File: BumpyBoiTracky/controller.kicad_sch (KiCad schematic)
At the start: 9 parts

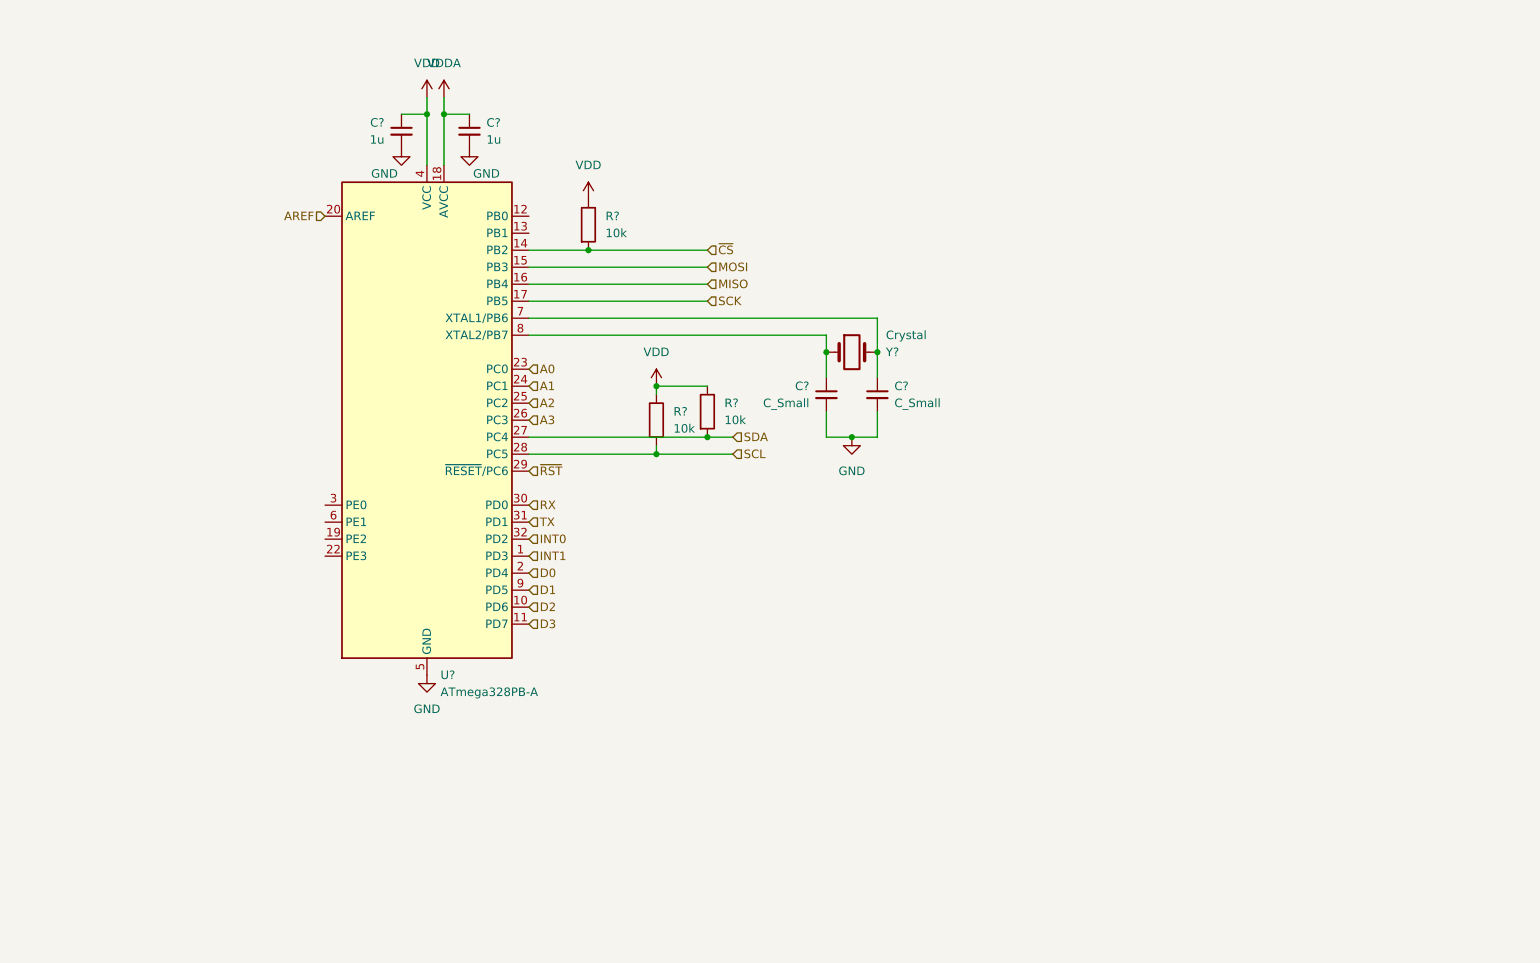
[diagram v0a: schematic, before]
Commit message: (adding forgotten files)
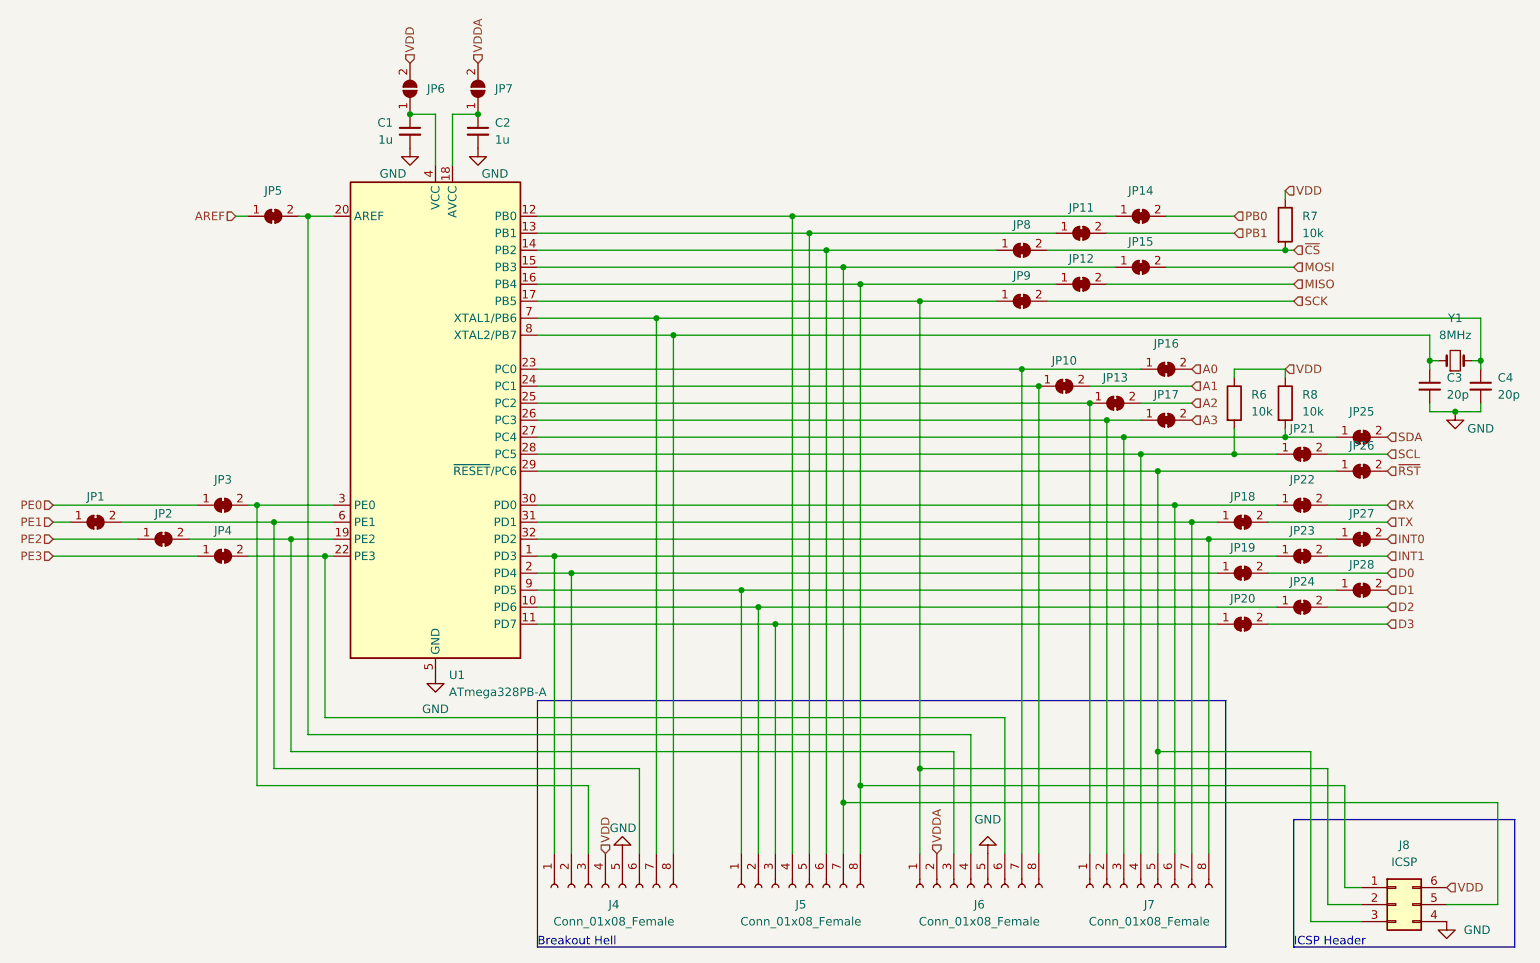
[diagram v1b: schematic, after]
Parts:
- removed C? (x2): C_Small, symbol Device:C_Small
- removed Y?: Crystal, symbol Device:Crystal
- added C3, C4: 20p, Capacitor_SMD:C_0603_1608Metric, symbol Device:C_Small
- added J4, J5, J6, J7: Conn_01x08_Female, Connector_PinHeader_2.54mm:PinHeader_1x08_P2.54mm_Vertical, symbol Connector:Conn_01x08_Female
- added J8: ICSP, Connector_PinHeader_2.54mm:PinHeader_2x03_P2.54mm_Vertical, symbol Connector_Generic:Conn_02x03_Counter_Clockwise
- added JP1, JP10, JP11, JP12, JP13, JP14, JP15, JP16, JP17, JP18, JP19, JP2, JP20, JP21, JP22, JP23, JP24, JP25, JP26, JP27, JP28, JP3, JP4, JP5, JP8, JP9: SolderJumper_2_Bridged, Jumper:SolderJumper-2_P1.3mm_Bridged_RoundedPad1.0x1.5mm, symbol Jumper:SolderJumper_2_Bridged
- added JP6, JP7: SolderJumper_2_Open, Jumper:SolderJumper-2_P1.3mm_Open_RoundedPad1.0x1.5mm, symbol Jumper:SolderJumper_2_Open
- added Y1: 8MHz, Crystal:Crystal_SMD_HC49-SD, symbol Device:Crystal_Small
- C1, C2: renamed from C?; footprint (none) -> Capacitor_SMD:C_0603_1608Metric
- R6, R7, R8: renamed from R?; footprint (none) -> Resistor_SMD:R_0603_1608Metric
- gave numbers to parts that had none: 1
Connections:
- net A0: now also JP16.2 (B); no longer U1.23 (PC0)
- net A1: now also JP10.2 (B); no longer U1.24 (PC1)
- net A2: now also JP13.2 (B); no longer U1.25 (PC2)
- net A3: now also JP17.2 (B); no longer U1.26 (PC3)
- net AREF: now also JP5.1 (A); no longer U1.20 (AREF)
- net D0: now also JP19.2 (B); no longer U1.2 (PD4)
- net D1: now also JP28.2 (B); no longer U1.9 (PD5)
- net D2: now also JP24.2 (B); no longer U1.10 (PD6)
- net D3: now also JP20.2 (B); no longer U1.11 (PD7)
- net GND: now also C3.2, C4.2, J4.5 (Pin_5), J6.5 (Pin_5), J8.4 (Pin_4)
- net INT0: now also JP27.2 (B); no longer U1.32 (PD2)
- net INT1: now also JP23.2 (B); no longer U1.1 (PD3)
- net MISO: now also JP12.2 (B); no longer U1.16 (PB4)
- net MOSI: now also JP15.2 (B); no longer U1.15 (PB3)
- net RX: now also JP22.2 (B); no longer U1.30 (PD0)
- net SCK: now also JP9.2 (B); no longer U1.17 (PB5)
- net SCL: now also JP21.2 (B); no longer R6.2, U1.28 (PC5)
- net SDA: now also JP25.2 (B); no longer R8.2, U1.27 (PC4)
- net TX: now also JP18.2 (B); no longer U1.31 (PD1)
- net VDD: now also J4.4 (Pin_4), J8.6 (Pin_6), JP6.2 (B); no longer C1.1, U1.4 (VCC)
- net VDDA: now also J6.2 (Pin_2), JP7.2 (B); no longer C2.1, U1.18 (AVCC)
- net ~{CS}: now also JP8.2 (B); no longer U1.14 (PB2)
- net ~{RST}: now also JP26.2 (B); no longer U1.29 (~{RESET}/PC6)
- net at U1.8 (XTAL2/PB7): now also C3.1, J4.8 (Pin_8), Y1.1
- net at U1.7 (XTAL1/PB6): now also C4.1, J4.7 (Pin_7), Y1.2
- net at U1.12 (PB0): now also J5.4 (Pin_4), JP14.1 (A)
- net at U1.13 (PB1): now also J5.5 (Pin_5), JP11.1 (A)
- net at U1.19 (PE2): now also J6.3 (Pin_3), JP2.2 (B)
- net at U1.22 (PE3): now also J6.6 (Pin_6), JP4.2 (B)
- net at U1.3 (PE0): now also J4.3 (Pin_3), JP3.2 (B)
- net at U1.6 (PE1): now also J4.6 (Pin_6), JP1.2 (B)
- new net: J7.7 (Pin_7), JP18.1 (A), U1.31 (PD1)
- new net: C1.1, JP6.1 (A), U1.4 (VCC)
- new net: J7.5 (Pin_5), J8.3 (Pin_3), JP26.1 (A), U1.29 (~{RESET}/PC6)
- new net: J6.1 (Pin_1), J8.2 (Pin_2), JP9.1 (A), U1.17 (PB5)
- new net: J5.8 (Pin_8), J8.1 (Pin_1), JP12.1 (A), U1.16 (PB4)
- new net: J5.7 (Pin_7), J8.5 (Pin_5), JP15.1 (A), U1.15 (PB3)
- new net: J7.1 (Pin_1), JP13.1 (A), U1.25 (PC2)
- new net: J7.2 (Pin_2), JP17.1 (A), U1.26 (PC3)
- new net: J7.3 (Pin_3), JP25.1 (A), R8.2, U1.27 (PC4)
- new net: J7.4 (Pin_4), JP21.1 (A), R6.2, U1.28 (PC5)
- new net: J7.6 (Pin_6), JP22.1 (A), U1.30 (PD0)
- new net: J7.8 (Pin_8), JP27.1 (A), U1.32 (PD2)
- new net: J6.4 (Pin_4), JP5.2 (B), U1.20 (AREF)
- new net: J6.7 (Pin_7), JP16.1 (A), U1.23 (PC0)
- new net: J5.1 (Pin_1), JP28.1 (A), U1.9 (PD5)
- new net: J5.2 (Pin_2), JP24.1 (A), U1.10 (PD6)
- new net: J5.3 (Pin_3), JP20.1 (A), U1.11 (PD7)
- new net: J5.6 (Pin_6), JP8.1 (A), U1.14 (PB2)
- new net: C2.1, JP7.1 (A), U1.18 (AVCC)
- new net: J4.1 (Pin_1), JP23.1 (A), U1.1 (PD3)
- new net: J4.2 (Pin_2), JP19.1 (A), U1.2 (PD4)
- new net: J6.8 (Pin_8), JP10.1 (A), U1.24 (PC1)
- new net PB0: JP14.2 (B)
- new net PB1: JP11.2 (B)
- new net PE0: JP3.1 (A)
- new net PE1: JP1.1 (A)
- new net PE2: JP2.1 (A)
- new net PE3: JP4.1 (A)
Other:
- note added: "Breakout Hell"
- note added: "ICSP Header"
- moved on the sheet: C1, C2, R6, R7, R8, U1
